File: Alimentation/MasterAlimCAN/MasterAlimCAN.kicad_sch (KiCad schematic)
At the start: 29 parts, among them J1 BATT, J10 Alim Log, J11 Alim 2, J13 Alim 3, U1 AMS1117-3.3, U2 STM32G474RETx, Y1 16MHz

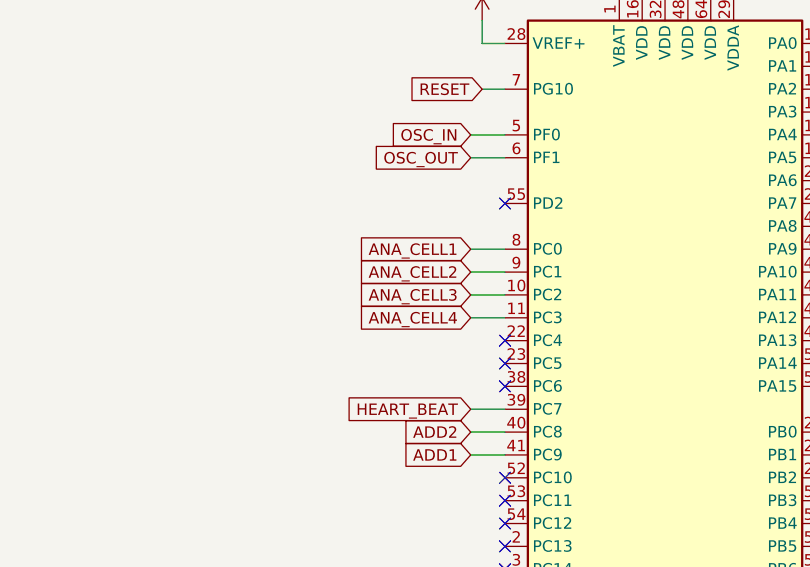
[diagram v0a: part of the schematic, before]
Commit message: Finish component placement on MasterAlimCAN
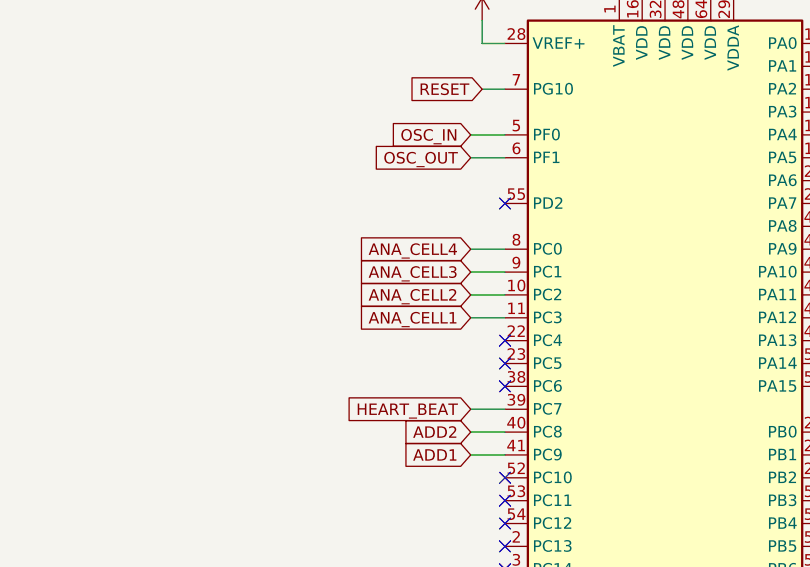
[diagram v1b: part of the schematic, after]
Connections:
- net ANA_CELL1: now also U2.11 (PC3); no longer U2.8 (PC0)
- net ANA_CELL2: now also U2.10 (PC2); no longer U2.9 (PC1)
- net ANA_CELL3: now also U2.9 (PC1); no longer U2.10 (PC2)
- net ANA_CELL4: now also U2.8 (PC0); no longer U2.11 (PC3)
